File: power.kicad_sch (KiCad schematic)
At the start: 18 parts, among them J2 USB_C_Receptacle_USB2.0_16P, J3 Conn_01x02_Pin, U4 USBLC6-2SC6, U5 BQ24090DGQ, U6 MAX17048G, U7 TPS7A0508PDBZ

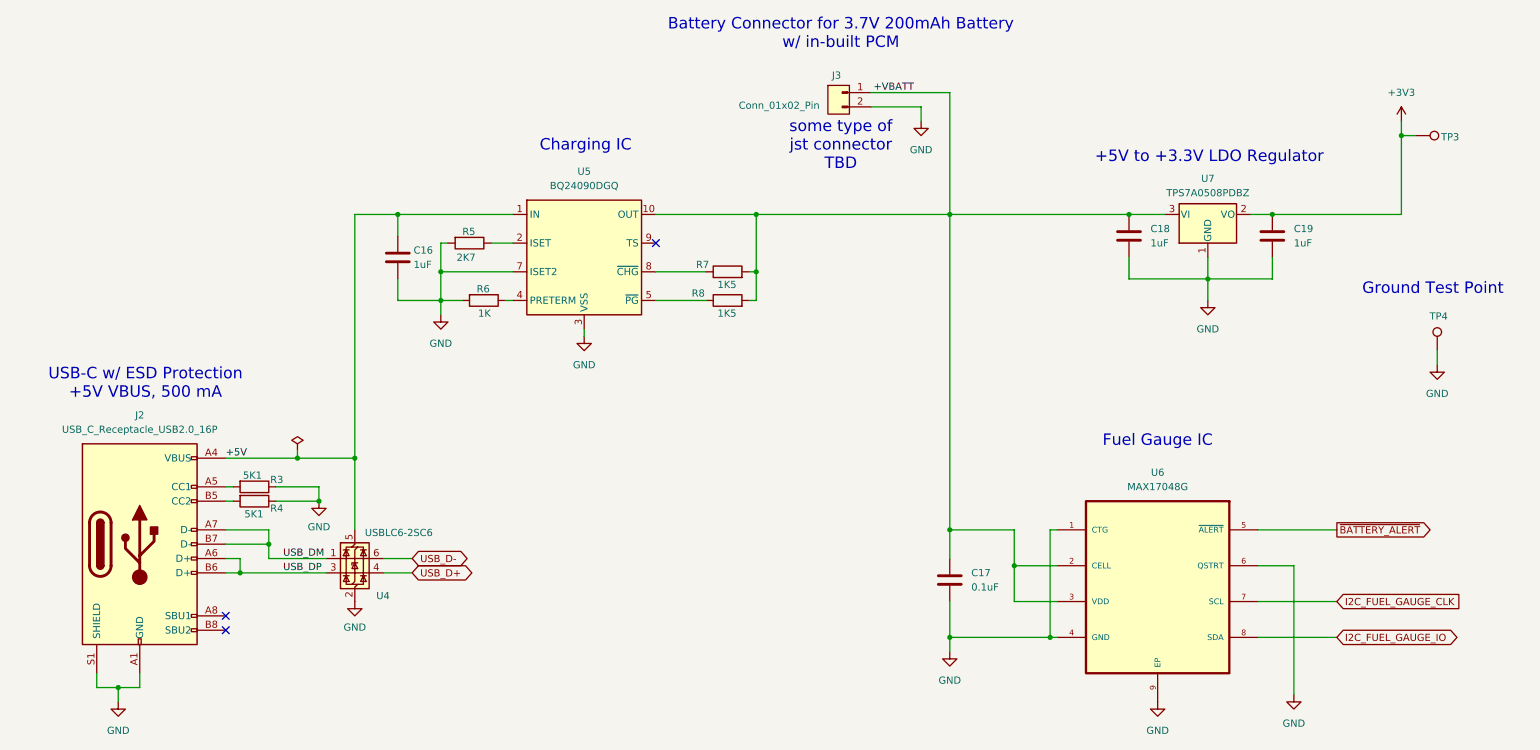
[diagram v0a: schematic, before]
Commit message: Layout progress
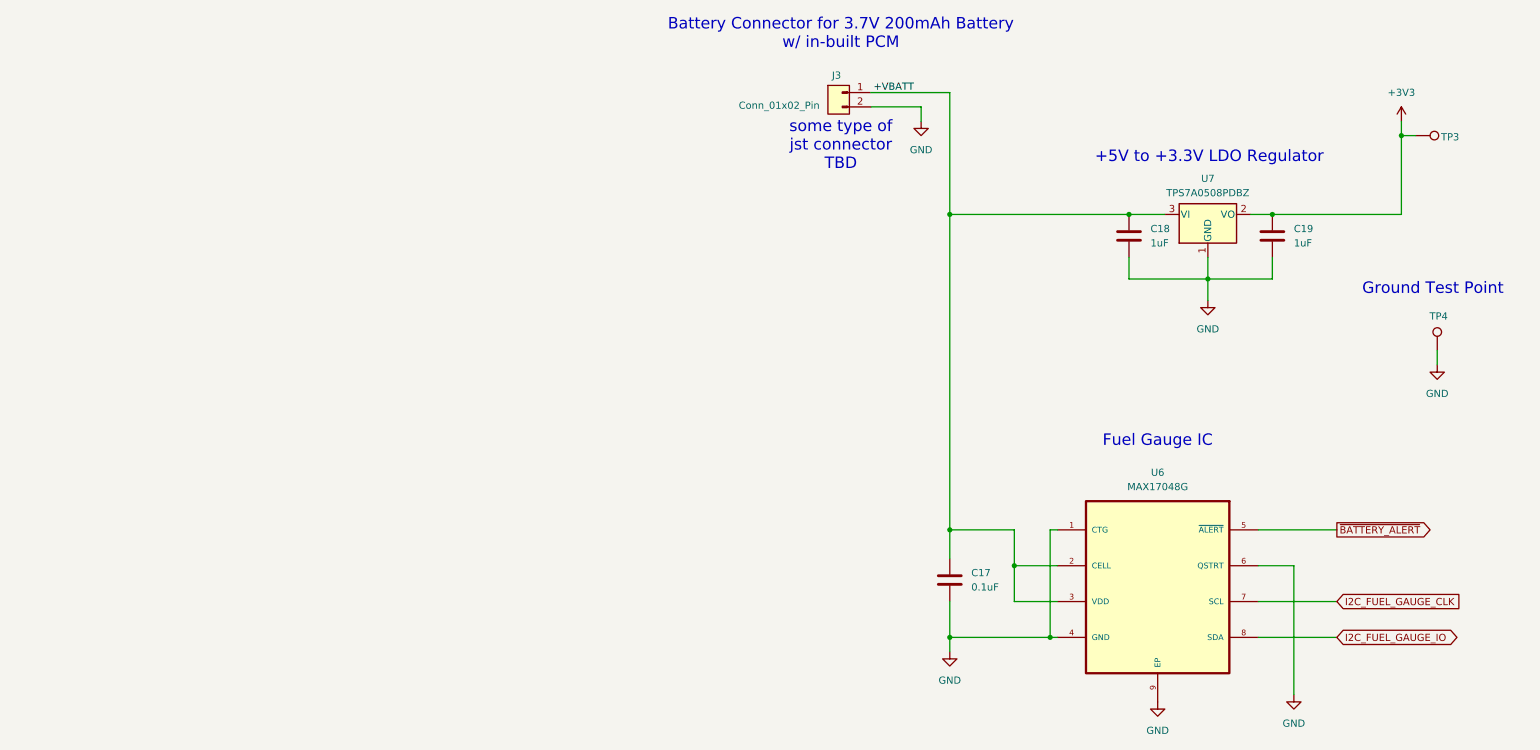
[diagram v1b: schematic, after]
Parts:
- removed C16: 1uF, Capacitor_SMD:C_0402_1005Metric, symbol Device:C
- removed J2: USB_C_Receptacle_USB2.0_16P, Connector_USB:USB_C_Receptacle_Molex_105450-0101, symbol Connector:USB_C_Receptacle_USB2.0_16P
- removed R3, R4: 5K1, Resistor_SMD:R_0402_1005Metric, symbol Device:R
- removed R5: 2K7, Resistor_SMD:R_0402_1005Metric, symbol Device:R
- removed R6: 1K, Resistor_SMD:R_0402_1005Metric, symbol Device:R
- removed R7, R8: 1K5, Resistor_SMD:R_0402_1005Metric, symbol Device:R
- removed U4: USBLC6-2SC6, Package_TO_SOT_SMD:SOT-23-6, symbol Power_Protection:USBLC6-2SC6
- removed U5: BQ24090DGQ, Package_SO:HVSSOP-10-1EP_3x3mm_P0.5mm_EP1.83x1.89mm, symbol Battery_Management:BQ24090DGQ
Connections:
- no-connect marks 3 -> 0
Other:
- note removed: "Charging IC"
- note removed: "USB-C w/ ESD Protection +5V VBUS, 500 mA"
